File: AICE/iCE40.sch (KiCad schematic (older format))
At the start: 5 parts

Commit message: Add files via upload
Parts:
- removed U?: W25Q128JVS, Package_SO:SOIC-8_5.23x5.23mm_P1.27mm, symbol Memory_Flash:W25Q128JVS
- added R? (x3): R, symbol Device:R
- added U?: W25Q, symbol w25q:W25Q
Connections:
- net labels added: Om_SPI0, Om_SPI1, Om_SPI2, Om_SPI3, Om_SPI4, Om_SPI[4,0], iCE_MISO, iCE_MOSI, iCE_SCLK, iCE_SS
- net labels removed: Om_SPI[3,0], SPI0, SPI1, SPI2, SPI3
- wire segments 9 -> 25
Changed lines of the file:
@@
 Wire Wire Line
 	1300 7550 1800 7550
-Text HLabel 2100 6900 0    50   BiDi ~ 0
-Om_SPI[3,0]
+Text HLabel 2100 6800 0    50   BiDi ~ 0
+Om_SPI[4,0]
 Wire Bus Line
-	2100 6900 2250 6900
-Entry Wire Line
-	2250 7450 2350 7550
+	2100 6800 2250 6800
 Entry Wire Line
 	2250 7350 2350 7450
@@
 Entry Wire Line
 	2250 7150 2350 7250
-Wire Wire Line
-	2350 7250 2850 7250
-Wire Wire Line
-	2350 7350 2850 7350
-Wire Wire Line
-	2350 7450 2850 7450
-Wire Wire Line
-	2350 7550 2850 7550
-Wire Bus Line
-	2250 6900 2250 7450
-Wire Bus Line
-	1200 6900 1200 7450
+Entry Wire Line
+	2250 7050 2350 7150
+Text Label 2350 7150 0    50   ~ 0
+Om_SPI0
 Text Label 2350 7250 0    50   ~ 0
-SPI0
+Om_SPI1
 Text Label 2350 7350 0    50   ~ 0
-SPI1
+Om_SPI2
 Text Label 2350 7450 0    50   ~ 0
-SPI2
-Text Label 2350 7550 0    50   ~ 0
-SPI3
+Om_SPI3
 Text Label 1300 7150 0    50   ~ 0
 COMM0
@@
 COMM4
 $Comp
-L Memory_Flash:W25Q128JVS U?
-U 1 1 5E904339
-P 9450 5200
-F 0 "U?" H 9450 5781 50  0000 C CNN
-F 1 "W25Q128JVS" H 9450 5690 50  0000 C CNN
-F 2 "Package_SO:SOIC-8_5.23x5.23mm_P1.27mm" H 9450 5200 50  0001 C CNN
-F 3 "http://www.winbond.com/resource-files/w25q128jv_dtr%20revc%2003272018%20plus.pdf" H 9450 5200 50  0001 C CNN
-	1    9450 5200
+L w25q:W25Q U?
+U 1 1 5E861C02
+P 8800 5150
+F 0 "U?" H 8800 5625 50  0000 C CNN
+F 1 "W25Q" H 8800 5534 50  0000 C CNN
+F 2 "" H 8800 5250 50  0001 C CNN
+F 3 "" H 8800 5250 50  0001 C CNN
+	1    8800 5150
 	1    0    0    -1
 $EndComp
+Wire Wire Line
+	6700 3900 7100 3900
+Wire Wire Line
+	6700 4000 7100 4000
+Wire Wire Line
+	6700 4100 7100 4100
+Wire Wire Line
+	6700 4200 7100 4200
+Text Label 7100 3900 2    50   ~ 0
+iCE_MISO
+Text Label 7100 4000 2    50   ~ 0
+iCE_MOSI
+Text Label 7100 4100 2    50   ~ 0
+iCE_SCLK
+Text Label 7100 4200 2    50   ~ 0
+iCE_SS
+Entry Wire Line
+	2250 7450 2350 7550
+Wire Wire Line
+	2350 7550 2850 7550
+Text Label 2350 7550 0    50   ~ 0
+Om_SPI4
+Text Label 3100 7150 2    50   ~ 0
+iCE_MISO
+Text Label 3100 7350 2    50   ~ 0
+iCE_MOSI
+Text Label 3100 7250 2    50   ~ 0
+iCE_SCLK
+Text Label 3100 7450 2    50   ~ 0
+iCE_SS
+Wire Wire Line
+	2350 7150 3100 7150
+Wire Wire Line
+	2350 7250 3100 7250
+Wire Wire Line
+	2350 7350 3100 7350
+Wire Wire Line
+	2350 7450 3100 7450
+Wire Wire Line
+	9200 5000 9650 5000
+Wire Wire Line
+	9200 5100 9650 5100
+Wire Wire Line
+	9200 5200 9650 5200
+Wire Wire Line
+	9200 5400 9650 5400
+Text Label 9650 5000 2    50   ~ 0
+iCE_SCLK
+Text Label 9650 5100 2    50   ~ 0
+iCE_MISO
+Text Label 9650 5200 2    50   ~ 0
+iCE_MOSI
+Text Label 9650 4900 2    50   ~ 0
+iCE_SS
+$Comp
+L Device:R R?
+U 1 1 5E89BD86
+P 9650 5600
+F 0 "R?" H 9720 5646 50  0000 L CNN
+F 1 "R" H 9720 5555 50  0000 L CNN
+F 2 "" V 9580 5600 50  0001 C CNN
+F 3 "~" H 9650 5600 50  0001 C CNN
+	1    9650 5600
+	1    0    0    -1
+$EndComp
+$Comp
+L Device:R R?
+U 1 1 5E89D2A2
+P 9900 5600
+F 0 "R?" H 9970 5646 50  0000 L CNN
+F 1 "R" H 9970 5555 50  0000 L CNN
+F 2 "" V 9830 5600 50  0001 C CNN
+F 3 "~" H 9900 5600 50  0001 C CNN
+	1    9900 5600
+	1    0    0    -1
+$EndComp
+Wire Wire Line
+	9650 5400 9650 5450
+Wire Wire Line
+	9900 5300 9900 5450
+Wire Wire Line
+	9200 5300 9900 5300
+Wire Wire Line
+	9650 5750 9650 5900
+Wire Wire Line
+	9650 5900 9900 5900
+Wire Wire Line
+	9900 5900 9900 5750
+$Comp
+L Device:R R?
+U 1 1 5E89EE9F
+P 9900 4750
+F 0 "R?" H 9970 4796 50  0000 L CNN
+F 1 "R" H 9970 4705 50  0000 L CNN
+F 2 "" V 9830 4750 50  0001 C CNN
+F 3 "~" H 9900 4750 50  0001 C CNN
+	1    9900 4750
+	1    0    0    -1
+$EndComp
+Wire Wire Line
+	9200 4900 9900 4900
+Wire Bus Line
+	1200 6900 1200 7450
+Wire Bus Line
+	2250 6800 2250 7450
 $EndSCHEMATC

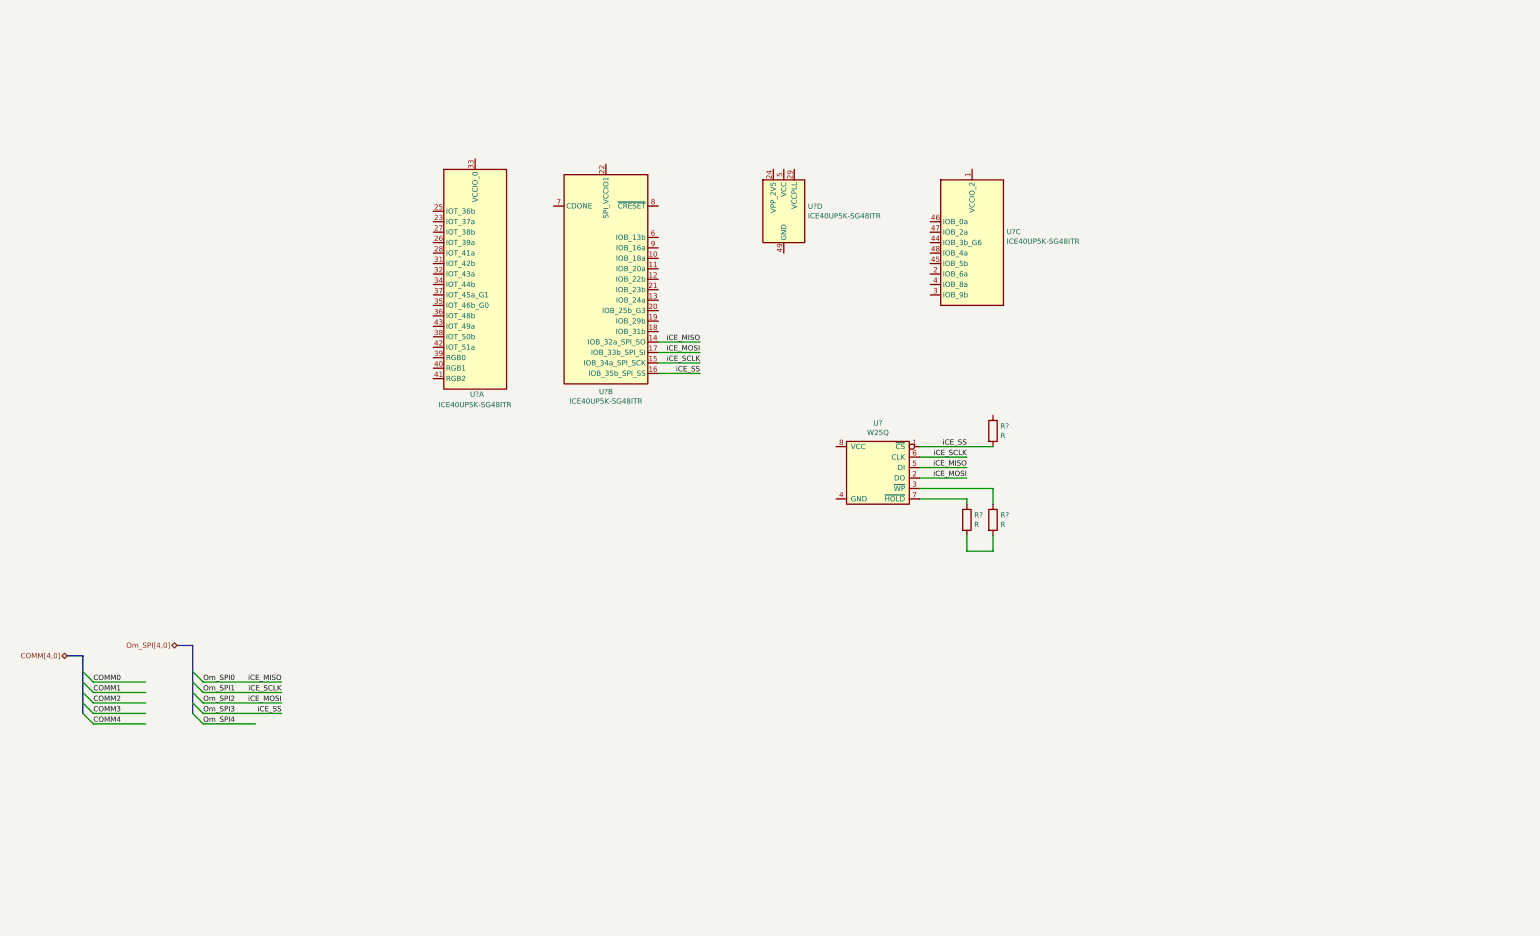
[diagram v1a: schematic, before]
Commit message: Add files via upload
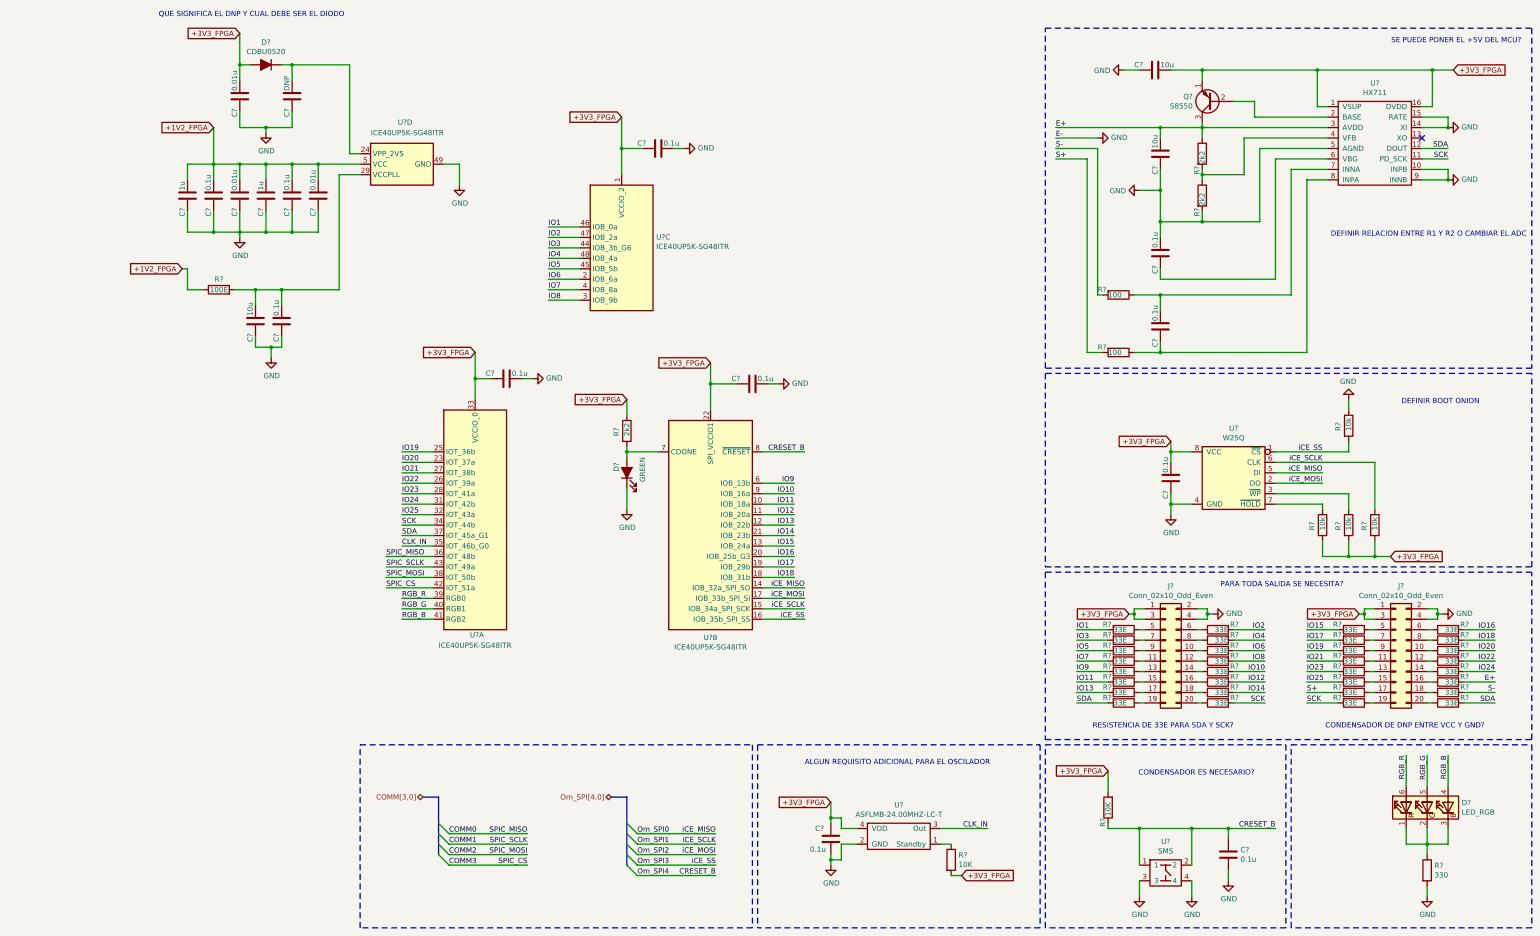
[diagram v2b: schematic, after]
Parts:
- removed R?: R, symbol Device:R
- added C? (x2): 1u, symbol Device:C
- added C? (x11): 0.1u, symbol Device:C
- added C? (x3): 0.01u, symbol Device:C
- added C?: DNP, symbol Device:C
- added C? (x3): 10u, symbol Device:C
- added D?: CDBU0520, symbol Device:D_ALT
- added D?: GREEN, symbol Device:LED_ALT
- added D?: LED_RGB, symbol Device:LED_RGB
- added J? (x2): Conn_02x10_Odd_Even, symbol Connector_Generic:Conn_02x10_Odd_Even
- added Q?: S8550, Package_TO_SOT_THT:TO-92_Inline, symbol Transistor_BJT:S8550
- added R?: 100E, symbol Device:R
- added R? (x3): 2k2, symbol Device:R
- added R? (x2): 10K, symbol Device:R
- added R? (x2): 100, symbol Device:R
- added R? (x2): 10k, symbol Device:R
- added R? (x32): 33E, symbol Device:R
- added R?: 330, symbol Device:R
- added U?: HX711, symbol ADC:HX711
- added U?: ASFLMB-24.00MHZ-LC-T, symbol OSC:ASFLMB-24.00MHZ-LC-T
- added U?: SMS, symbol pulse:SMS
- R? (x2): value R -> 10k
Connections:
- net labels added: +1V2_FPGA, +3V3_FPGA, CLK_IN, COMM[3,0], CRESET_B, E+, E-, GND, IO1, IO10, IO11, IO12, IO13, IO14, IO15, IO16, IO17, IO18, IO19, IO2, IO20, IO21, IO22, IO23, IO24, IO25, IO3, IO4, IO5, IO6, IO7, IO8, IO9, RGB_B, RGB_G, RGB_R, S+, S-, SCK, SDA, SPIC_CS, SPIC_MISO, SPIC_MOSI, SPIC_SCLK
- net labels removed: COMM4, COMM[4,0]
- wire segments 25 -> 325
- no-connect marks 0 -> 1
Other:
- note added: "ALGUN REQUISITO ADICIONAL PARA EL OSCILADOR"
- note added: "CONDENSADOR DE DNP ENTRE VCC Y GND?"
- note added: "CONDENSADOR ES NECESARIO?"
- note added: "DEFINIR BOOT ONION"
- note added: "DEFINIR RELACION ENTRE R1 Y R2 O CAMBIAR EL ADC"
- note added: "PARA TODA SALIDA SE NECESITA?"
- note added: "QUE SIGNIFICA EL DNP Y CUAL DEBE SER EL DIODO"
- note added: "RESISTENCIA DE 33E PARA SDA Y SCK?"
- note added: "SE PUEDE PONER EL +5V DEL MCU?"
- moved on the sheet: R?, U?, U?A, U?B, U?C, U?D
